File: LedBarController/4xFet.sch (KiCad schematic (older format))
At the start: 4 parts, among them Q301 Si2302DS, Q302 Si2302DS, Q303 Si2302DS, Q304 Si2302DS

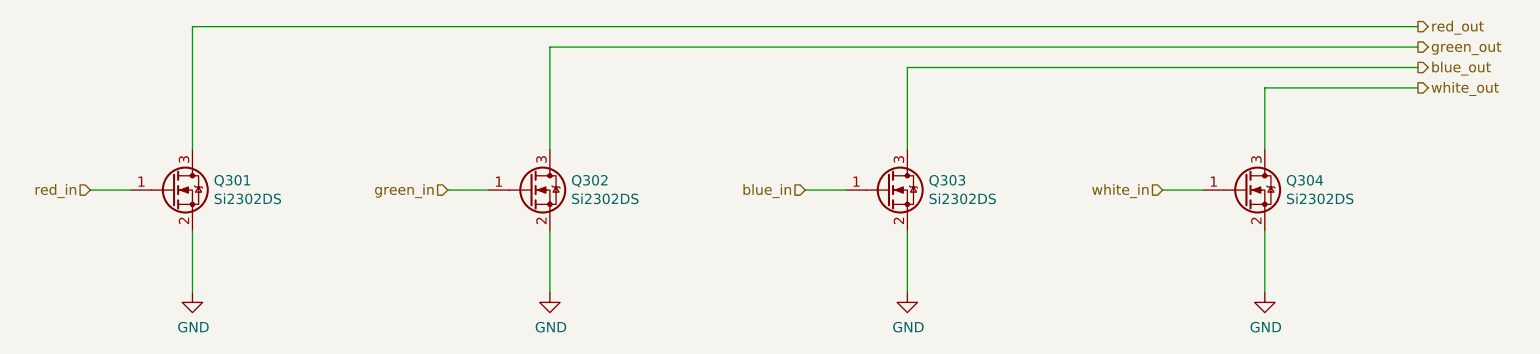
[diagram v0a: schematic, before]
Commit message: Route complete
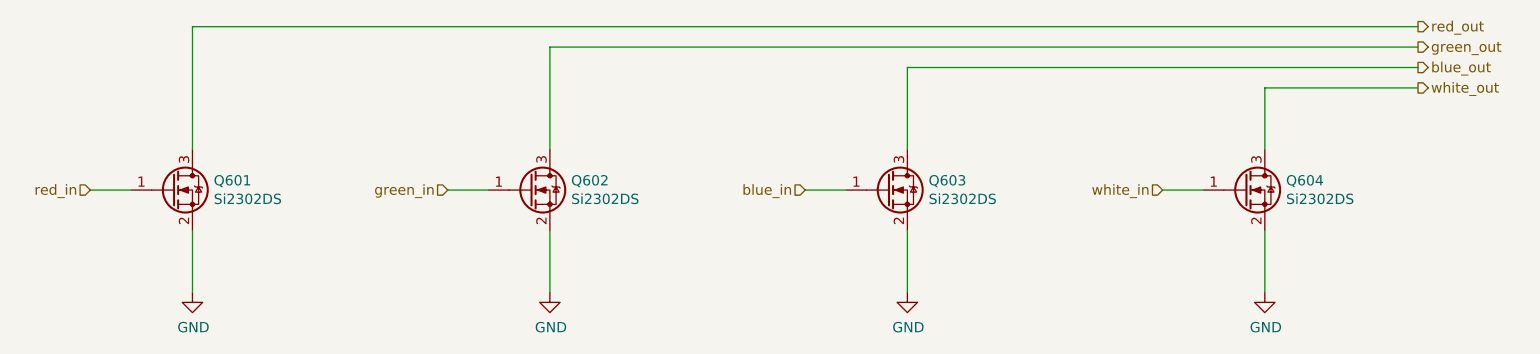
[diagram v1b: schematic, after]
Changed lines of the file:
@@
 $Descr A4 11693 8268
 encoding utf-8
-Sheet 3 13
+Sheet 6 13
 Title ""
 Date ""
@@
 AR Path="/5F8F2E1B/5F902D83/5F88FE81" Ref="Q504"  Part="1"
 AR Path="/5F8F2E1B/5F902E61/5F88FE81" Ref="Q604"  Part="1"
-F 0 "Q304" H 7854 3846 50  0000 L CNN
+F 0 "Q604" H 7854 3846 50  0000 L CNN
 F 1 "Si2302DS" H 7854 3755 50  0000 L CNN
 F 2 "Package_TO_SOT_SMD:SOT-23_Handsoldering" H 7850 3900 50  0001 C CNN
@@
 AR Path="/5F8F2E1B/5F902D83/5F88FE73" Ref="Q503"  Part="1"
 AR Path="/5F8F2E1B/5F902E61/5F88FE73" Ref="Q603"  Part="1"
-F 0 "Q303" H 6104 3846 50  0000 L CNN
+F 0 "Q603" H 6104 3846 50  0000 L CNN
 F 1 "Si2302DS" H 6104 3755 50  0000 L CNN
 F 2 "Package_TO_SOT_SMD:SOT-23_Handsoldering" H 6100 3900 50  0001 C CNN
@@
 AR Path="/5F8F2E1B/5F902D83/5F88FE65" Ref="Q502"  Part="1"
 AR Path="/5F8F2E1B/5F902E61/5F88FE65" Ref="Q602"  Part="1"
-F 0 "Q302" H 4354 3846 50  0000 L CNN
+F 0 "Q602" H 4354 3846 50  0000 L CNN
 F 1 "Si2302DS" H 4354 3755 50  0000 L CNN
 F 2 "Package_TO_SOT_SMD:SOT-23_Handsoldering" H 4350 3900 50  0001 C CNN
@@
 AR Path="/5F8F2E1B/5F902D83/5F88FE58" Ref="Q501"  Part="1"
 AR Path="/5F8F2E1B/5F902E61/5F88FE58" Ref="Q601"  Part="1"
-F 0 "Q301" H 2604 3846 50  0000 L CNN
+F 0 "Q601" H 2604 3846 50  0000 L CNN
 F 1 "Si2302DS" H 2604 3755 50  0000 L CNN
 F 2 "Package_TO_SOT_SMD:SOT-23_Handsoldering" H 2600 3900 50  0001 C CNN

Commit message: Added AT24C256
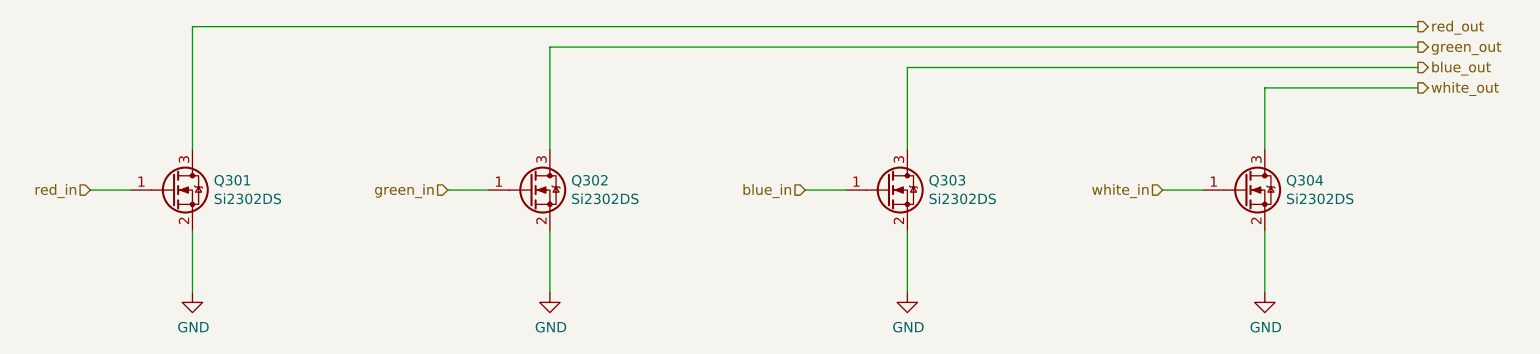
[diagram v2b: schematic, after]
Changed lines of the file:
@@
 $Descr A4 11693 8268
 encoding utf-8
-Sheet 6 13
+Sheet 3 13
 Title ""
 Date ""
@@
 AR Path="/5F8F2E1B/5F902D83/5F88FE81" Ref="Q504"  Part="1"
 AR Path="/5F8F2E1B/5F902E61/5F88FE81" Ref="Q604"  Part="1"
-F 0 "Q604" H 7854 3846 50  0000 L CNN
+F 0 "Q304" H 7854 3846 50  0000 L CNN
 F 1 "Si2302DS" H 7854 3755 50  0000 L CNN
 F 2 "Package_TO_SOT_SMD:SOT-23_Handsoldering" H 7850 3900 50  0001 C CNN
@@
 AR Path="/5F8F2E1B/5F902D83/5F88FE73" Ref="Q503"  Part="1"
 AR Path="/5F8F2E1B/5F902E61/5F88FE73" Ref="Q603"  Part="1"
-F 0 "Q603" H 6104 3846 50  0000 L CNN
+F 0 "Q303" H 6104 3846 50  0000 L CNN
 F 1 "Si2302DS" H 6104 3755 50  0000 L CNN
 F 2 "Package_TO_SOT_SMD:SOT-23_Handsoldering" H 6100 3900 50  0001 C CNN
@@
 AR Path="/5F8F2E1B/5F902D83/5F88FE65" Ref="Q502"  Part="1"
 AR Path="/5F8F2E1B/5F902E61/5F88FE65" Ref="Q602"  Part="1"
-F 0 "Q602" H 4354 3846 50  0000 L CNN
+F 0 "Q302" H 4354 3846 50  0000 L CNN
 F 1 "Si2302DS" H 4354 3755 50  0000 L CNN
 F 2 "Package_TO_SOT_SMD:SOT-23_Handsoldering" H 4350 3900 50  0001 C CNN
@@
 AR Path="/5F8F2E1B/5F902D83/5F88FE58" Ref="Q501"  Part="1"
 AR Path="/5F8F2E1B/5F902E61/5F88FE58" Ref="Q601"  Part="1"
-F 0 "Q601" H 2604 3846 50  0000 L CNN
+F 0 "Q301" H 2604 3846 50  0000 L CNN
 F 1 "Si2302DS" H 2604 3755 50  0000 L CNN
 F 2 "Package_TO_SOT_SMD:SOT-23_Handsoldering" H 2600 3900 50  0001 C CNN
